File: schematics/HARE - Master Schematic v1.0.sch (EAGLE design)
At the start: 109 parts, among them IC1 NE5532N, IC2 NE5532N, IC3 FT232RL, IC4 NE5532N, IC5 7805DT, IC6 TM1804IS62/65WVS0648, J1 9V, J2 STEREOSW, J3 STEREOSW, Q1 16 MHz, SW2 Reset Button, U1 ATMEGA328P-PU, U2 MCP4921-E/P, X2 USB-B-H

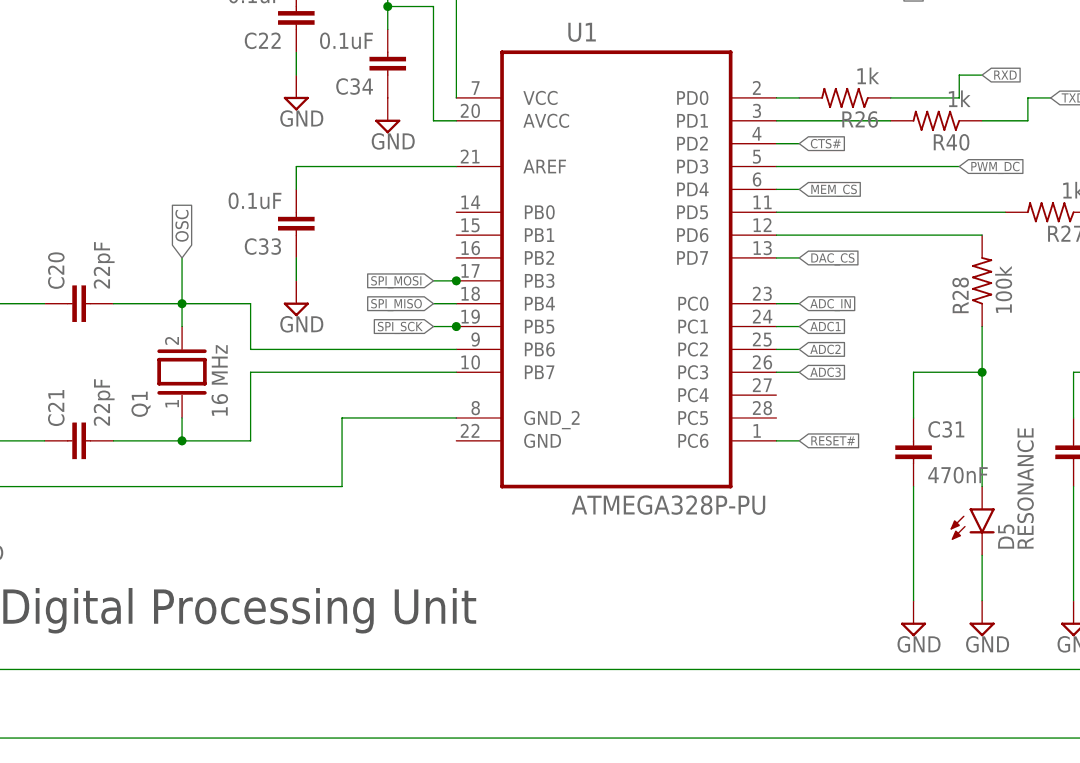
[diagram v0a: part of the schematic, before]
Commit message: REV 1 for HARE ready for tapeout
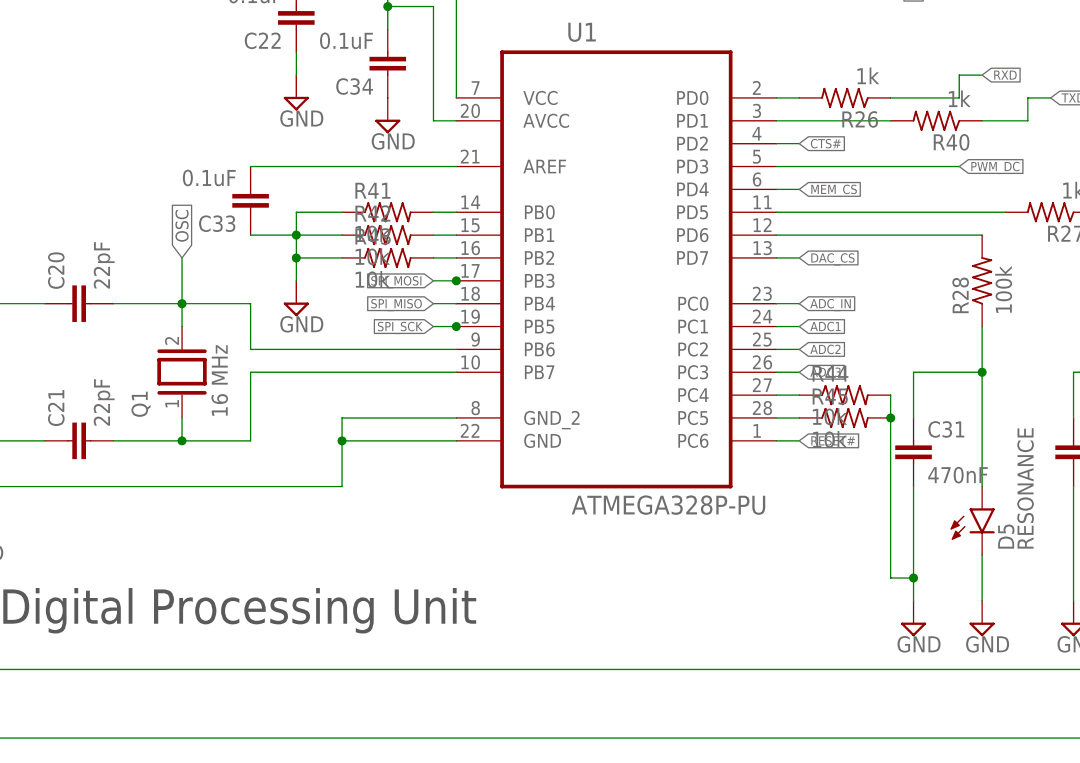
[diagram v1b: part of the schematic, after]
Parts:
- added R41, R42, R43, R44, R45: 10k, resistor:R-US_R0805
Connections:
- new net N$39: R41.2, U1.PB0
- new net N$44: R42.2, U1.PB1
- new net N$47: R43.2, U1.PB2
- new net N$50: R44.1, U1.PC4
- new net N$55: R45.1, U1.PC5
- net GND: now also R41.1, R42.1, R43.1, R44.2, R45.2, U1.GND
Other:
- moved on the sheet: C33
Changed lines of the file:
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@@
 <part name="R40" library="resistor" library_urn="urn:adsk.eagle:library:348" deviceset="R-US_" device="R0805" package3d_urn="urn:adsk.eagle:package:26059/1" value="1k"/>
 <part name="C37" library="resistor" library_urn="urn:adsk.eagle:library:348" deviceset="C-EU" device="C0805K" package3d_urn="urn:adsk.eagle:package:26201/1" value="10uF"/>
+<part name="R41" library="resistor" library_urn="urn:adsk.eagle:library:348" deviceset="R-US_" device="R0805" package3d_urn="urn:adsk.eagle:package:26059/1" value="10k"/>
+<part name="R42" library="resistor" library_urn="urn:adsk.eagle:library:348" deviceset="R-US_" device="R0805" package3d_urn="urn:adsk.eagle:package:26059/1" value="10k"/>
+<part name="R43" library="resistor" library_urn="urn:adsk.eagle:library:348" deviceset="R-US_" device="R0805" package3d_urn="urn:adsk.eagle:package:26059/1" value="10k"/>
+<part name="R44" library="resistor" library_urn="urn:adsk.eagle:library:348" deviceset="R-US_" device="R0805" package3d_urn="urn:adsk.eagle:package:26059/1" value="10k"/>
+<part name="R45" library="resistor" library_urn="urn:adsk.eagle:library:348" deviceset="R-US_" device="R0805" package3d_urn="urn:adsk.eagle:package:26059/1" value="10k"/>
 </parts>
 <sheets>
@@
 <instance part="C31" gate="G$1" x="129.54" y="314.96"/>
 <instance part="C32" gate="G$1" x="147.32" y="314.96"/>
-<instance part="C33" gate="G$1" x="60.96" y="340.36" rot="R180"/>
+<instance part="C33" gate="G$1" x="55.88" y="342.9" rot="R180"/>
 <instance part="SUPPLY47" gate="GND" x="60.96" y="332.74"/>
 <instance part="C34" gate="G$1" x="71.12" y="358.14" rot="R180"/>
@@
 <instance part="R40" gate="G$1" x="132.08" y="353.06" rot="R180"/>
 <instance part="C37" gate="G$1" x="137.16" y="383.54" rot="R180"/>
+<instance part="R41" gate="G$1" x="71.12" y="342.9"/>
+<instance part="R42" gate="G$1" x="71.12" y="340.36"/>
+<instance part="R43" gate="G$1" x="71.12" y="337.82"/>
+<instance part="R44" gate="G$1" x="121.92" y="322.58"/>
+<instance part="R45" gate="G$1" x="121.92" y="320.04"/>
 </instances>
 <busses>
@@
 <pinref part="U1" gate="A" pin="GND_2"/>
 <wire x1="78.74" y1="320.04" x2="66.04" y2="320.04" width="0.1524" layer="91"/>
-<wire x1="66.04" y1="320.04" x2="66.04" y2="312.42" width="0.1524" layer="91"/>
+<wire x1="66.04" y1="320.04" x2="66.04" y2="317.5" width="0.1524" layer="91"/>
+<wire x1="66.04" y1="317.5" x2="66.04" y2="312.42" width="0.1524" layer="91"/>
 <wire x1="66.04" y1="312.42" x2="25.4" y2="312.42" width="0.1524" layer="91"/>
 <junction x="25.4" y="312.42"/>
+<pinref part="U1" gate="A" pin="GND"/>
+<wire x1="78.74" y1="317.5" x2="66.04" y2="317.5" width="0.1524" layer="91"/>
+<junction x="66.04" y="317.5"/>
 </segment>
 <segment>
@@
 <pinref part="C31" gate="G$1" pin="2"/>
 <pinref part="SUPPLY46" gate="GND" pin="GND"/>
-<wire x1="129.54" y1="312.42" x2="129.54" y2="299.72" width="0.1524" layer="91"/>
+<wire x1="129.54" y1="312.42" x2="129.54" y2="302.26" width="0.1524" layer="91"/>
+<wire x1="129.54" y1="302.26" x2="129.54" y2="299.72" width="0.1524" layer="91"/>
+<wire x1="127" y1="322.58" x2="127" y2="320.04" width="0.1524" layer="91"/>
+<wire x1="127" y1="320.04" x2="127" y2="302.26" width="0.1524" layer="91"/>
+<wire x1="127" y1="302.26" x2="129.54" y2="302.26" width="0.1524" layer="91"/>
+<junction x="129.54" y="302.26"/>
+<pinref part="R44" gate="G$1" pin="2"/>
+<pinref part="R45" gate="G$1" pin="2"/>
+<junction x="127" y="320.04"/>
 </segment>
 <segment>
@@
 <pinref part="C33" gate="G$1" pin="1"/>
 <wire x1="60.96" y1="335.28" x2="60.96" y2="337.82" width="0.1524" layer="91"/>
+<wire x1="60.96" y1="337.82" x2="60.96" y2="340.36" width="0.1524" layer="91"/>
+<wire x1="60.96" y1="340.36" x2="55.88" y2="340.36" width="0.1524" layer="91"/>
+<pinref part="R41" gate="G$1" pin="1"/>
+<wire x1="66.04" y1="342.9" x2="60.96" y2="342.9" width="0.1524" layer="91"/>
+<wire x1="60.96" y1="342.9" x2="60.96" y2="340.36" width="0.1524" layer="91"/>
+<junction x="60.96" y="340.36"/>
+<pinref part="R42" gate="G$1" pin="1"/>
+<wire x1="66.04" y1="340.36" x2="60.96" y2="340.36" width="0.1524" layer="91"/>
+<pinref part="R43" gate="G$1" pin="1"/>
+<wire x1="66.04" y1="337.82" x2="60.96" y2="337.82" width="0.1524" layer="91"/>
+<junction x="60.96" y="337.82"/>
 </segment>
 <segment>
@@
 <segment>
 <pinref part="C33" gate="G$1" pin="2"/>
-<wire x1="60.96" y1="345.44" x2="60.96" y2="347.98" width="0.1524" layer="91"/>
 <pinref part="U1" gate="A" pin="AREF"/>
-<wire x1="60.96" y1="347.98" x2="78.74" y2="347.98" width="0.1524" layer="91"/>
+<wire x1="55.88" y1="347.98" x2="78.74" y2="347.98" width="0.1524" layer="91"/>
 </segment>
 </net>
@@
 </segment>
 </net>
+<net name="N$39" class="0">
+<segment>
+<pinref part="U1" gate="A" pin="PB0"/>
+<pinref part="R41" gate="G$1" pin="2"/>
+<wire x1="78.74" y1="342.9" x2="76.2" y2="342.9" width="0.1524" layer="91"/>
+</segment>
+</net>
+<net name="N$44" class="0">
+<segment>
+<pinref part="U1" gate="A" pin="PB1"/>
+<pinref part="R42" gate="G$1" pin="2"/>
+<wire x1="78.74" y1="340.36" x2="76.2" y2="340.36" width="0.1524" layer="91"/>
+</segment>
+</net>
+<net name="N$47" class="0">
+<segment>
+<pinref part="U1" gate="A" pin="PB2"/>
+<pinref part="R43" gate="G$1" pin="2"/>
+<wire x1="78.74" y1="337.82" x2="76.2" y2="337.82" width="0.1524" layer="91"/>
+</segment>
+</net>
+<net name="N$50" class="0">
+<segment>
+<pinref part="U1" gate="A" pin="PC4"/>
+<pinref part="R44" gate="G$1" pin="1"/>
+<wire x1="116.84" y1="322.58" x2="114.3" y2="322.58" width="0.1524" layer="91"/>
+</segment>
+</net>
+<net name="N$55" class="0">
+<segment>
+<pinref part="U1" gate="A" pin="PC5"/>
+<pinref part="R45" gate="G$1" pin="1"/>
+<wire x1="116.84" y1="320.04" x2="114.3" y2="320.04" width="0.1524" layer="91"/>
+</segment>
+</net>
